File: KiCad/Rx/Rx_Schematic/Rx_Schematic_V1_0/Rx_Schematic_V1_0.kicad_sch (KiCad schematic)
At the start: 5 parts, among them J1 Analog, J2 Digital

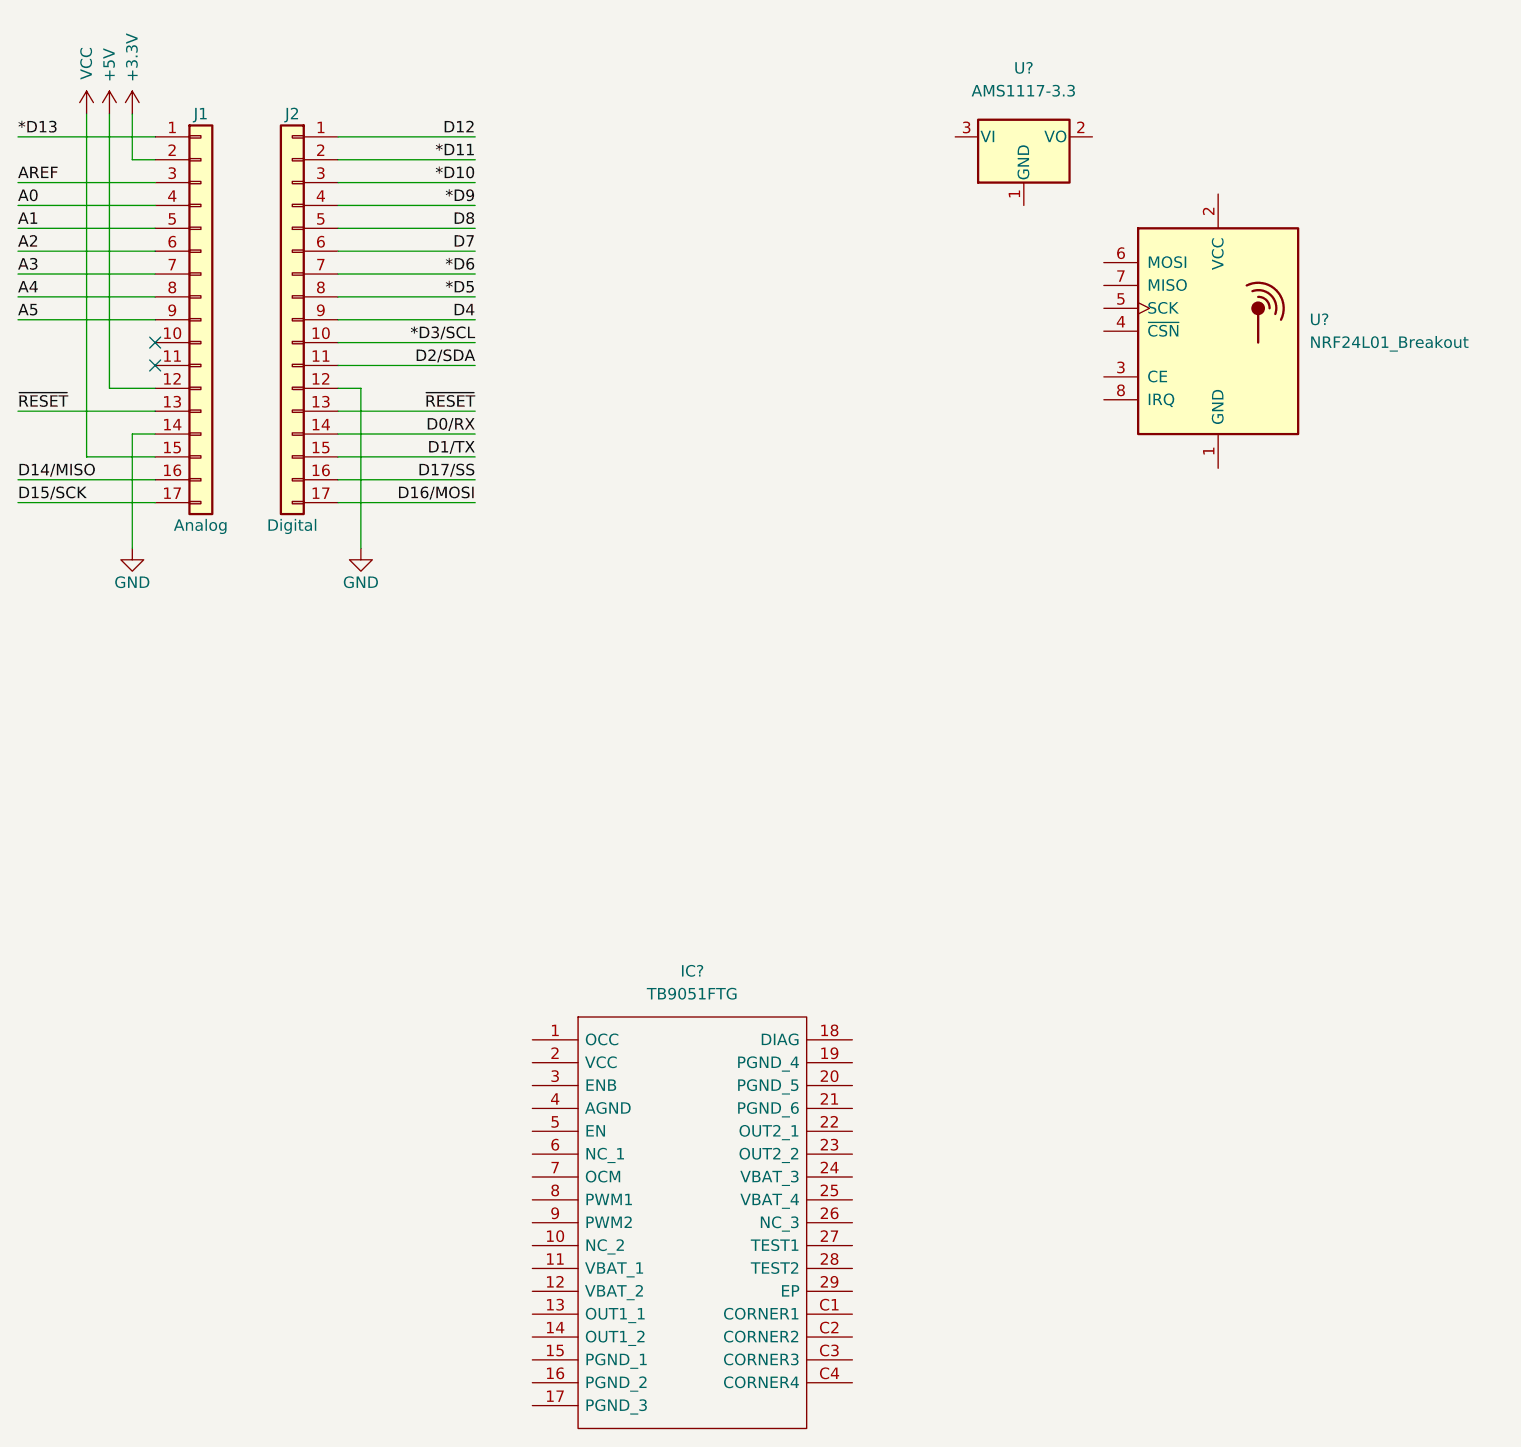
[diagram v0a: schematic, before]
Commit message: Updated schematic
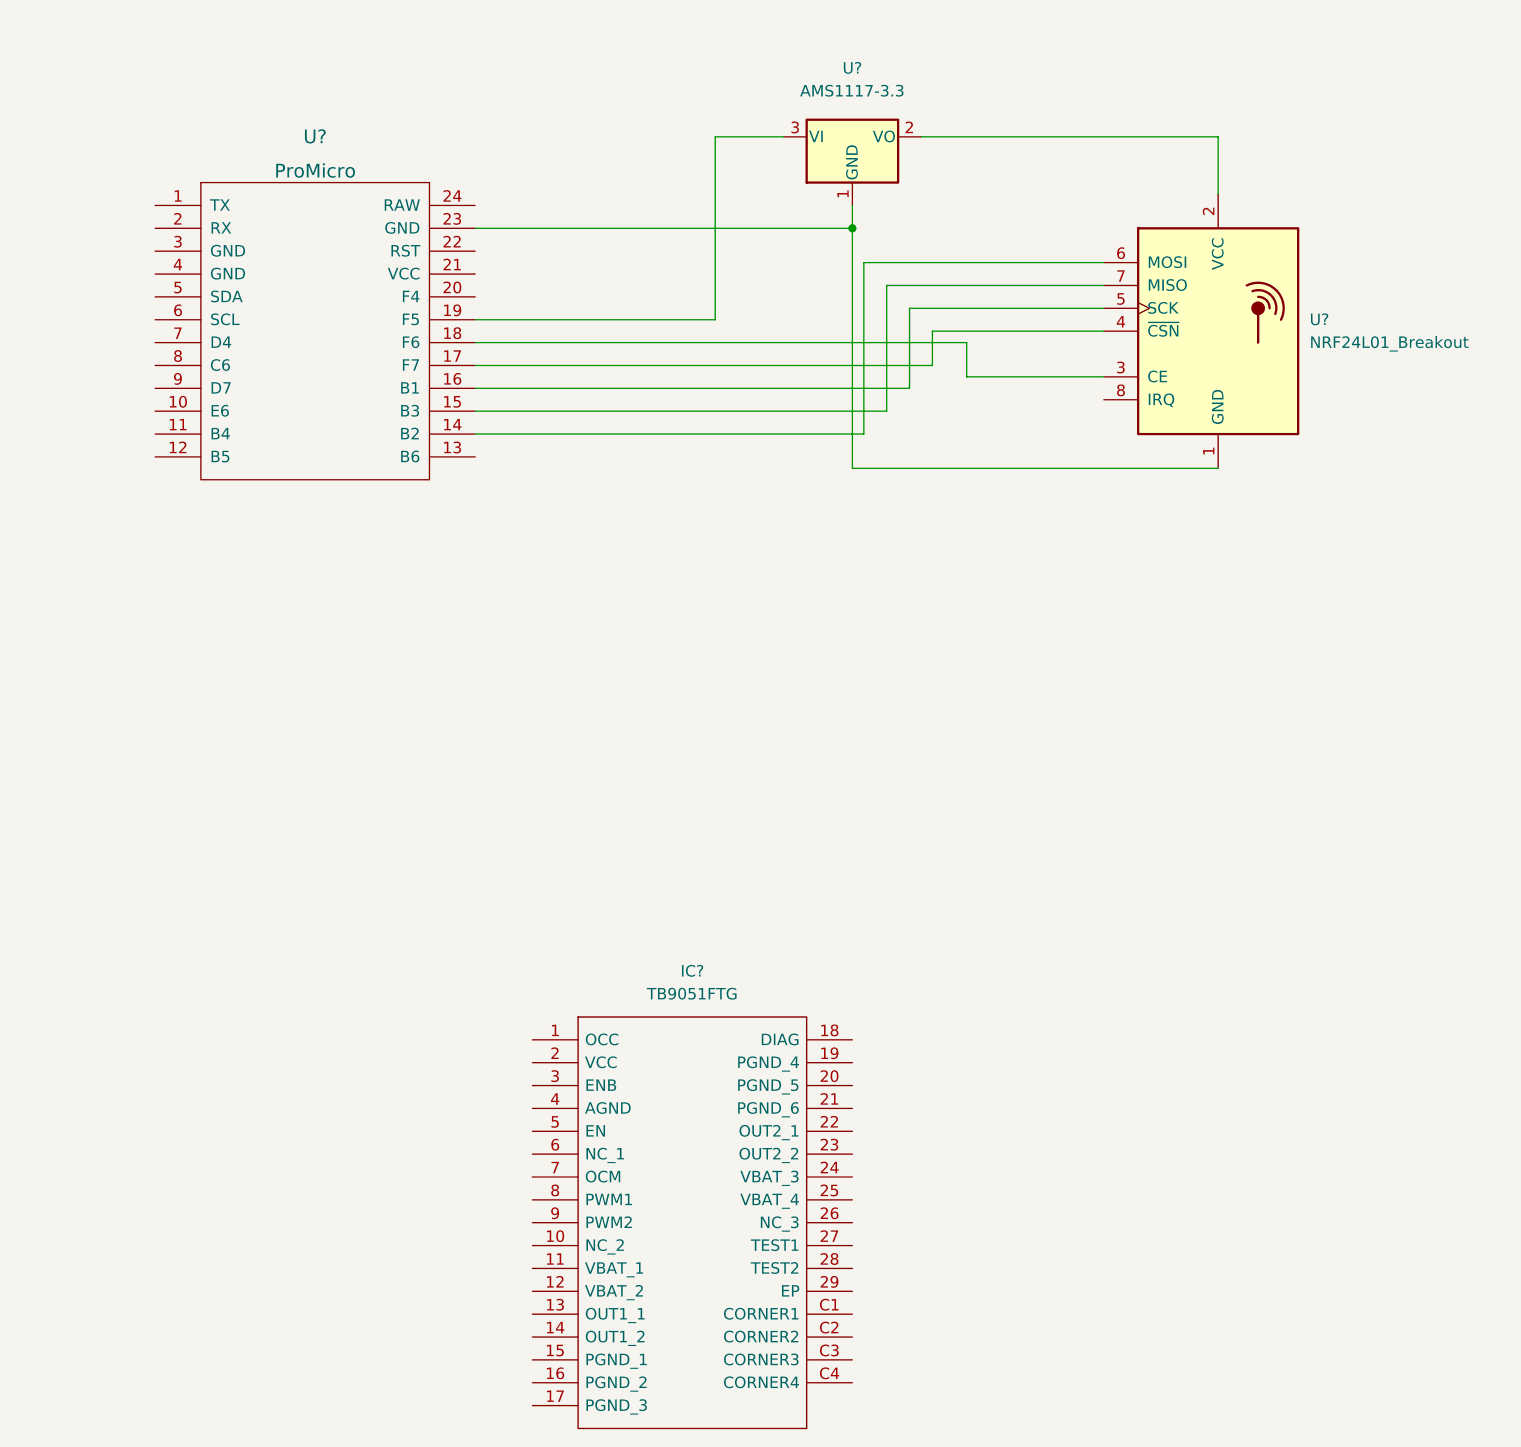
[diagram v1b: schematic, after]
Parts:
- removed J1: Analog, Connector_PinHeader_2.54mm:PinHeader_1x17_P2.54mm_Vertical, symbol Connector_Generic:Conn_01x17
- removed J2: Digital, Connector_PinHeader_2.54mm:PinHeader_1x17_P2.54mm_Vertical, symbol Connector_Generic:Conn_01x17
- added U?: ProMicro, symbol promicro:ProMicro
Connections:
- net at U?.1 (GND): now also U?.1 (GND), U?.23 (GND)
- net at U?.2 (VO): now also U?.2 (VCC)
- net at U?.3 (VI): now also U?.19 (F5)
- net at U?.3 (CE): now also U?.18 (F6)
- net at U?.4 (~{CSN}): now also U?.17 (F7)
- net at U?.5 (SCK): now also U?.16 (B1)
- net at U?.6 (MOSI): now also U?.14 (B2)
- net at U?.7 (MISO): now also U?.15 (B3)
- no-connect marks 2 -> 0
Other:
- moved on the sheet: U?
